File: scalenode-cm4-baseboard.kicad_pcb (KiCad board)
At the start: 4 copper layers, 128.5 x 40 mm, 147 parts, among them IC1 TPS2378DDA, J1 B2B-XH-A_LF__SN_, J10 LSHM-130-01-L-RH-A-S-K-TR, J3 1-2199230-6, J4 1140084168, J5 0473460001, J6 SS-74800-144, J7 DF40HC(3.0)-100DS-0.4v, J8 DF40HC(3.0)-100DS-0.4v, Q6 BSS138-7-F, U1 TS3USB30EDGSR, U2 AP62301WU-7, U3 TPS2373-3RGW, U4 URB4805YMD-30WR3, U5 TS3USB30EDGSR, U6 FT234XD-R

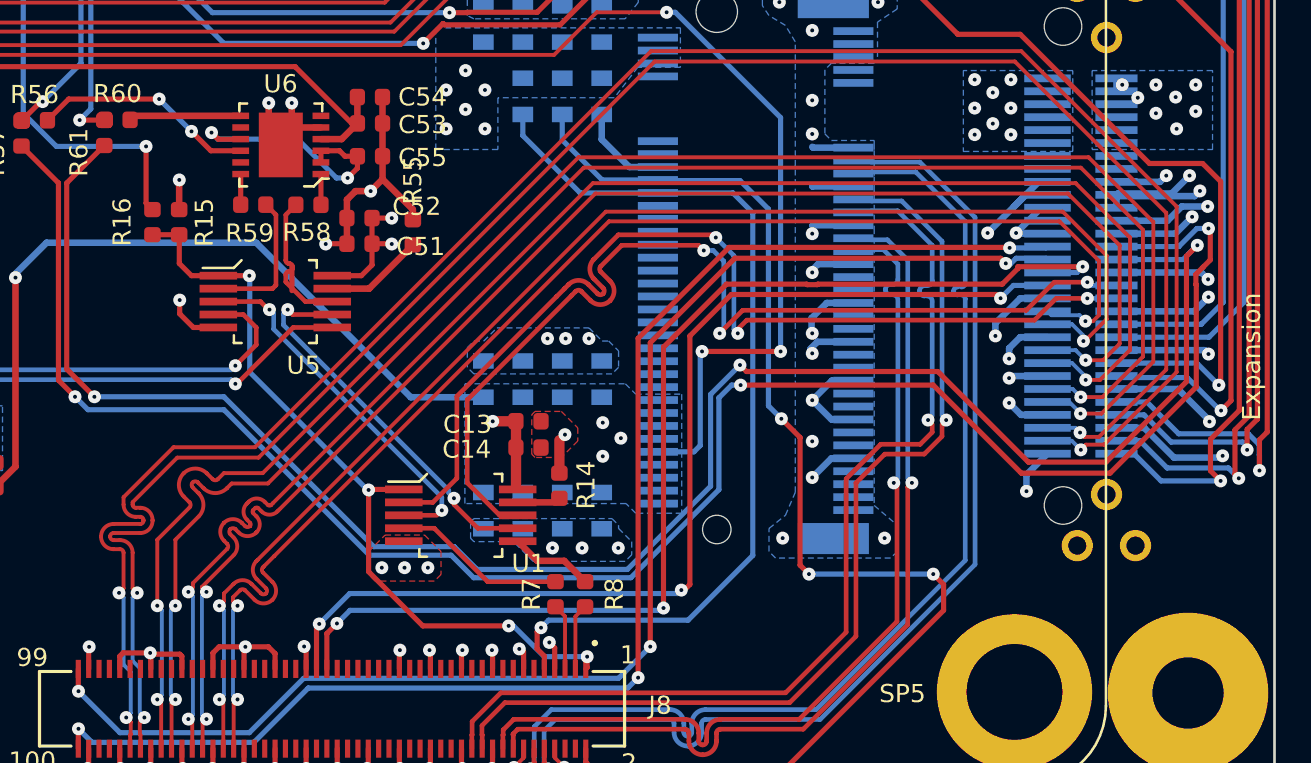
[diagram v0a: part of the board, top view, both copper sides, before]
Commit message: Guide tracks out of vias
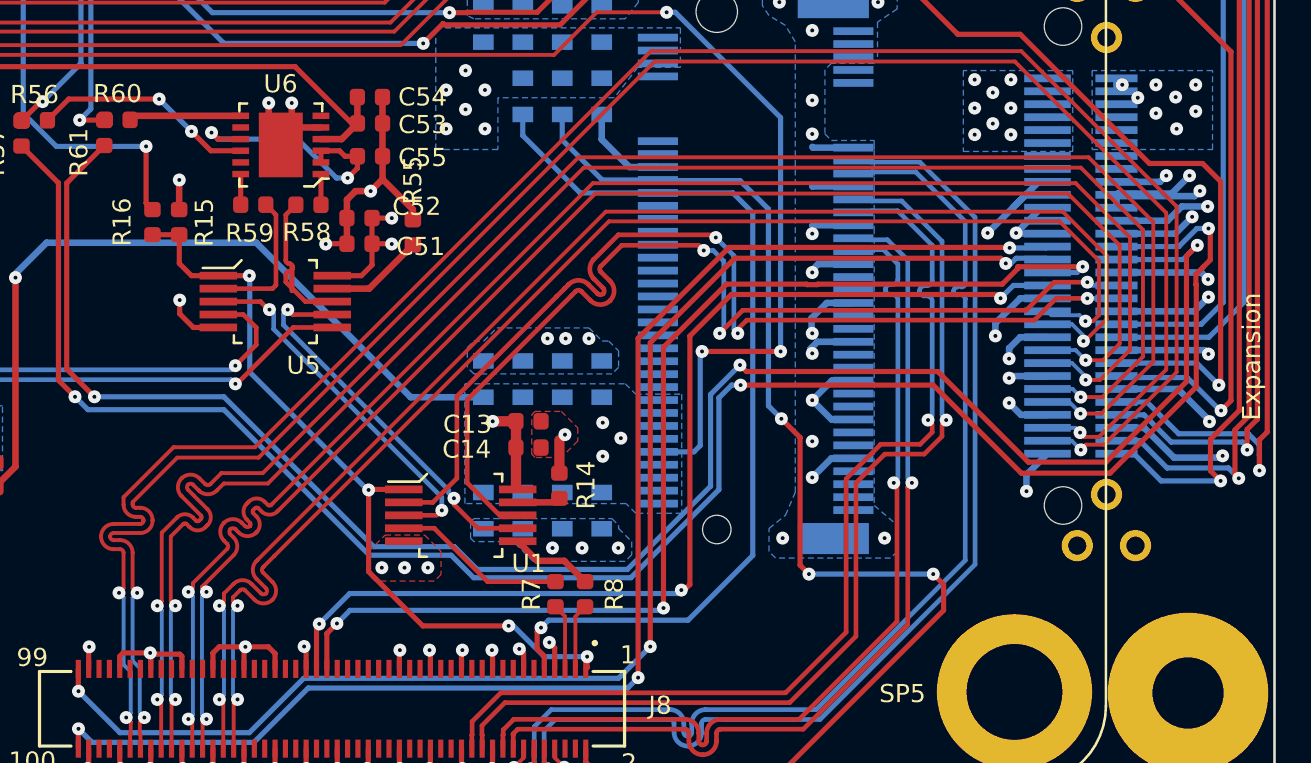
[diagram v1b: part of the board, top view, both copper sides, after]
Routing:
- net HDMI0_D0_P: track 64.0 -> 65.3 mm
- net HDMI0_D0_N: track 65.9 -> 66.9 mm
